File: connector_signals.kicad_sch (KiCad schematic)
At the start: 5 parts, among them J4 Conn_01x05, J5 Conn_01x05, J6 Conn_01x05, J7 Mega Connector/Breakout (if w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, P1 USB_C_Plug_USB2.0

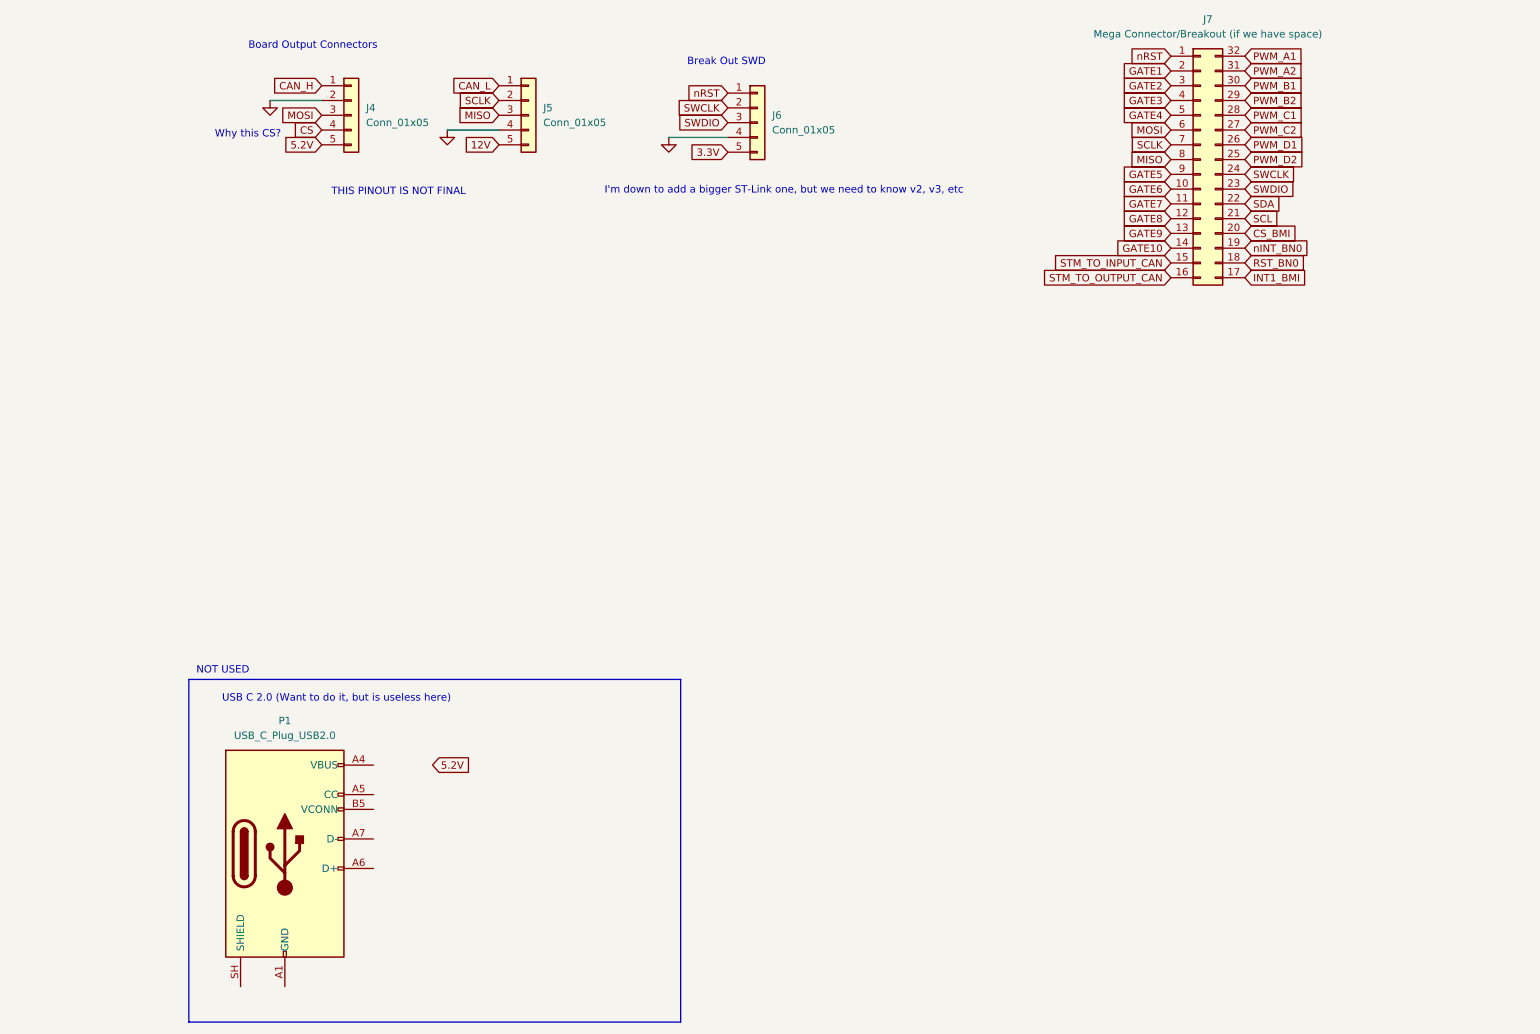
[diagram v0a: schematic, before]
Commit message: Commit for Milwaukee Review
Version 0.2 Completed
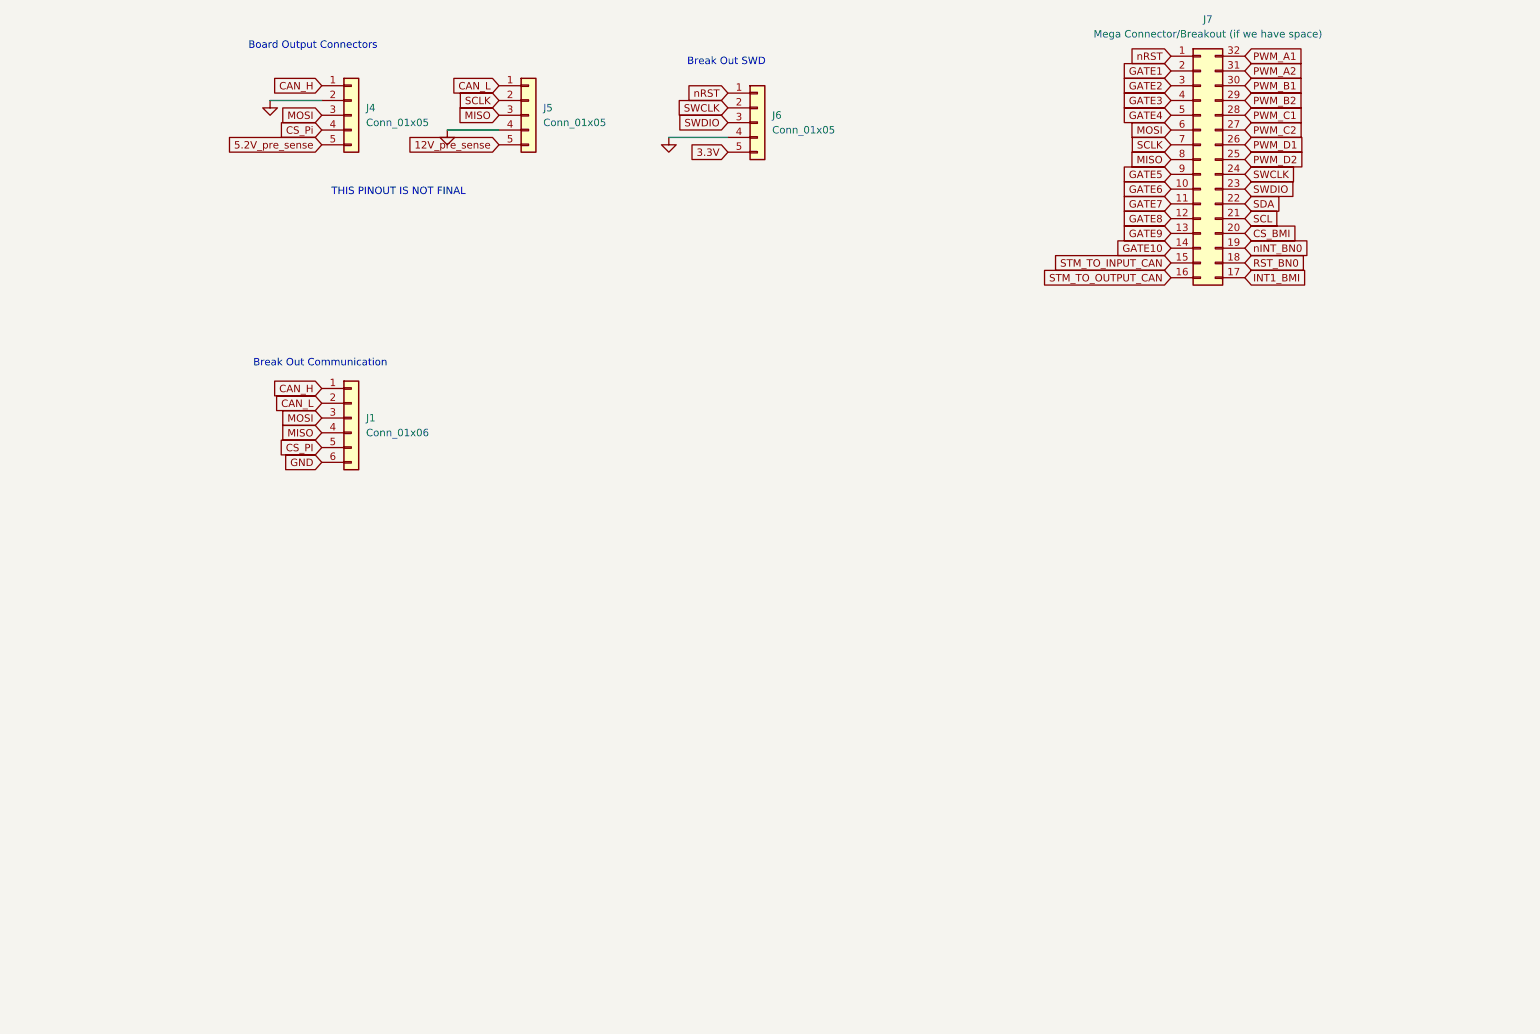
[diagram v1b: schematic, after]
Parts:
- removed P1: USB_C_Plug_USB2.0, symbol Connector:USB_C_Plug_USB2.0
- added J1: Conn_01x06, symbol Connector_Generic:Conn_01x06
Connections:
- net CAN_H: now also J1.1 (Pin_1)
- net CAN_L: now also J1.2 (Pin_2)
- net GND: now also J1.6 (Pin_6)
- net MISO: now also J1.4 (Pin_4)
- net MOSI: now also J1.3 (Pin_3)
- net 12V renamed 12V_pre_sense
- net 5.2V renamed 5.2V_pre_sense
- net CS renamed CS_Pi
- new net CS_PI: J1.5 (Pin_5)
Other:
- note added: "Break Out Communication"
- note removed: "I'm down to add a bigger ST-Link one, but we need to know v2, v3, etc"
- note removed: "NOT USED"
- note removed: "USB C 2.0 (Want to do it, but is useless here)"
- note removed: "Why this CS?"

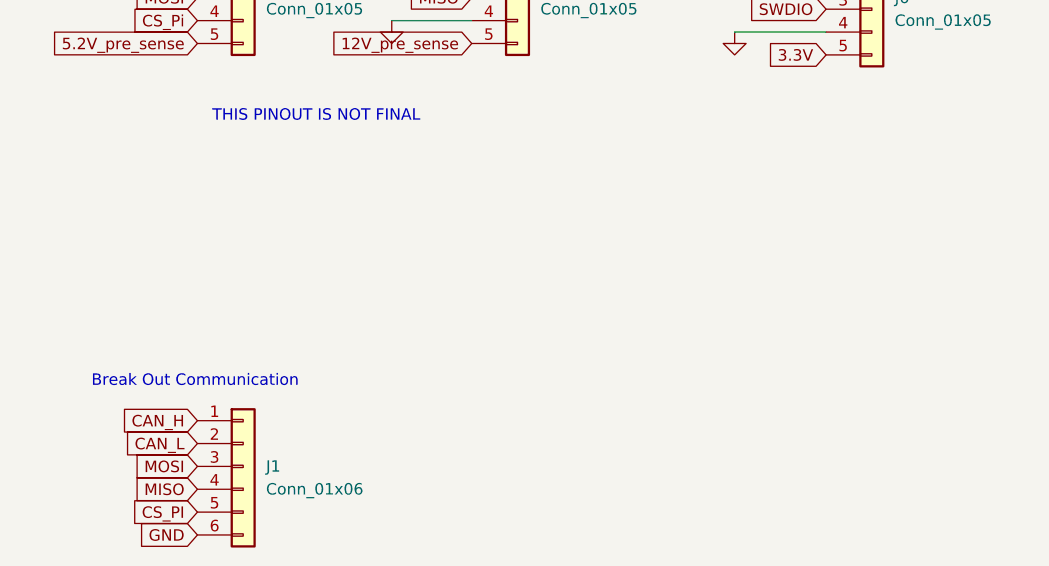
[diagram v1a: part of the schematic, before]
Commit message: Update ig
We messed up
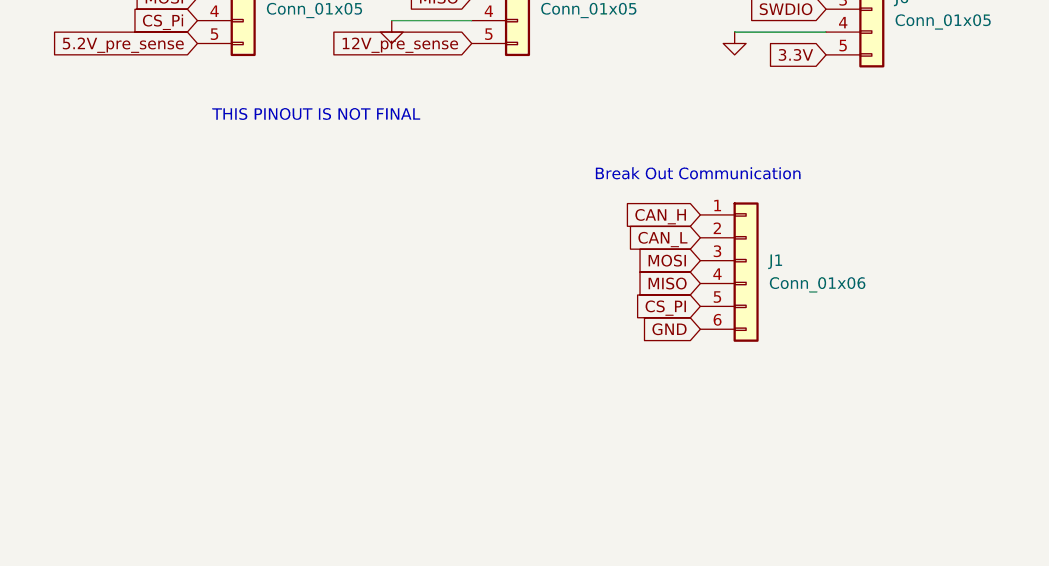
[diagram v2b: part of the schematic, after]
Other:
- moved on the sheet: J1
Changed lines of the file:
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@@
 	(text "Break Out Communication"
 		(exclude_from_sim no)
-		(at 41.656 78.232 0)
+		(at 97.536 55.372 0)
 		(effects
 			(font
@@
 	(global_label "CS_PI"
 		(shape input)
-		(at 41.91 92.71 180)
-		(fields_autoplaced yes)
-		(effects
-			(font
-				(size 1.27 1.27)
-			)
-			(justify right)
-		)
-		(property "Intersheetrefs" "${INTERSHEET_REFS}"
-			(at 33.6029 92.71 0)
+		(at 97.79 69.85 180)
+		(fields_autoplaced yes)
+		(effects
+			(font
+				(size 1.27 1.27)
+			)
+			(justify right)
+		)
+		(property "Intersheetrefs" "${INTERSHEET_REFS}"
+			(at 89.4829 69.85 0)
 			(hide yes)
 			(show_name no)
@@
 	(global_label "GND"
 		(shape input)
-		(at 41.91 95.25 180)
-		(fields_autoplaced yes)
-		(effects
-			(font
-				(size 1.27 1.27)
-			)
-			(justify right)
-		)
-		(property "Intersheetrefs" "${INTERSHEET_REFS}"
-			(at 35.0543 95.25 0)
+		(at 97.79 72.39 180)
+		(fields_autoplaced yes)
+		(effects
+			(font
+				(size 1.27 1.27)
+			)
+			(justify right)
+		)
+		(property "Intersheetrefs" "${INTERSHEET_REFS}"
+			(at 90.9343 72.39 0)
 			(hide yes)
 			(show_name no)
@@
 	(global_label "CAN_L"
 		(shape input)
-		(at 41.91 85.09 180)
-		(fields_autoplaced yes)
-		(effects
-			(font
-				(size 1.27 1.27)
-			)
-			(justify right)
-		)
-		(property "Intersheetrefs" "${INTERSHEET_REFS}"
-			(at 33.24 85.09 0)
+		(at 97.79 62.23 180)
+		(fields_autoplaced yes)
+		(effects
+			(font
+				(size 1.27 1.27)
+			)
+			(justify right)
+		)
+		(property "Intersheetrefs" "${INTERSHEET_REFS}"
+			(at 89.12 62.23 0)
 			(hide yes)
 			(show_name no)
@@
 	(global_label "CAN_H"
 		(shape input)
-		(at 41.91 82.55 180)
-		(fields_autoplaced yes)
-		(effects
-			(font
-				(size 1.27 1.27)
-			)
-			(justify right)
-		)
-		(property "Intersheetrefs" "${INTERSHEET_REFS}"
-			(at 32.9376 82.55 0)
+		(at 97.79 59.69 180)
+		(fields_autoplaced yes)
+		(effects
+			(font
+				(size 1.27 1.27)
+			)
+			(justify right)
+		)
+		(property "Intersheetrefs" "${INTERSHEET_REFS}"
+			(at 88.8176 59.69 0)
 			(hide yes)
 			(show_name no)
@@
 	(global_label "MOSI"
 		(shape input)
-		(at 41.91 87.63 180)
-		(fields_autoplaced yes)
-		(effects
-			(font
-				(size 1.27 1.27)
-			)
-			(justify right)
-		)
-		(property "Intersheetrefs" "${INTERSHEET_REFS}"
-			(at 34.3286 87.63 0)
+		(at 97.79 64.77 180)
+		(fields_autoplaced yes)
+		(effects
+			(font
+				(size 1.27 1.27)
+			)
+			(justify right)
+		)
+		(property "Intersheetrefs" "${INTERSHEET_REFS}"
+			(at 90.2086 64.77 0)
 			(hide yes)
 			(show_name no)
@@
 	(global_label "MISO"
 		(shape input)
-		(at 41.91 90.17 180)
-		(fields_autoplaced yes)
-		(effects
-			(font
-				(size 1.27 1.27)
-			)
-			(justify right)
-		)
-		(property "Intersheetrefs" "${INTERSHEET_REFS}"
-			(at 34.3286 90.17 0)
+		(at 97.79 67.31 180)
+		(fields_autoplaced yes)
+		(effects
+			(font
+				(size 1.27 1.27)
+			)
+			(justify right)
+		)
+		(property "Intersheetrefs" "${INTERSHEET_REFS}"
+			(at 90.2086 67.31 0)
 			(hide yes)
 			(show_name no)
@@
 	(symbol
 		(lib_id "Connector_Generic:Conn_01x06")
-		(at 46.99 87.63 0)
+		(at 102.87 64.77 0)
 		(unit 1)
 		(body_style 1)
@@
 		(fields_autoplaced yes)
 		(property "Reference" "J1"
-			(at 49.53 87.6299 0)
+			(at 105.41 64.7699 0)
 			(show_name no)
 			(do_not_autoplace no)
@@
 		)
 		(property "Value" "Conn_01x06"
-			(at 49.53 90.1699 0)
+			(at 105.41 67.3099 0)
 			(show_name no)
 			(do_not_autoplace no)
@@
 		)
 		(property "Footprint" ""
-			(at 46.99 87.63 0)
+			(at 102.87 64.77 0)
 			(hide yes)
 			(show_name no)
@@
 		)
 		(property "Datasheet" ""
-			(at 46.99 87.63 0)
+			(at 102.87 64.77 0)
 			(hide yes)
 			(show_name no)
@@
 		)
 		(property "Description" "Generic connector, single row, 01x06, script generated (kicad-library-utils/schlib/autogen/connector/)"
-			(at 46.99 87.63 0)
-			(hide yes)
-			(show_name no)
+			(at 102.87 64.77 0)
+			(hide yes)
+			(show_name no)

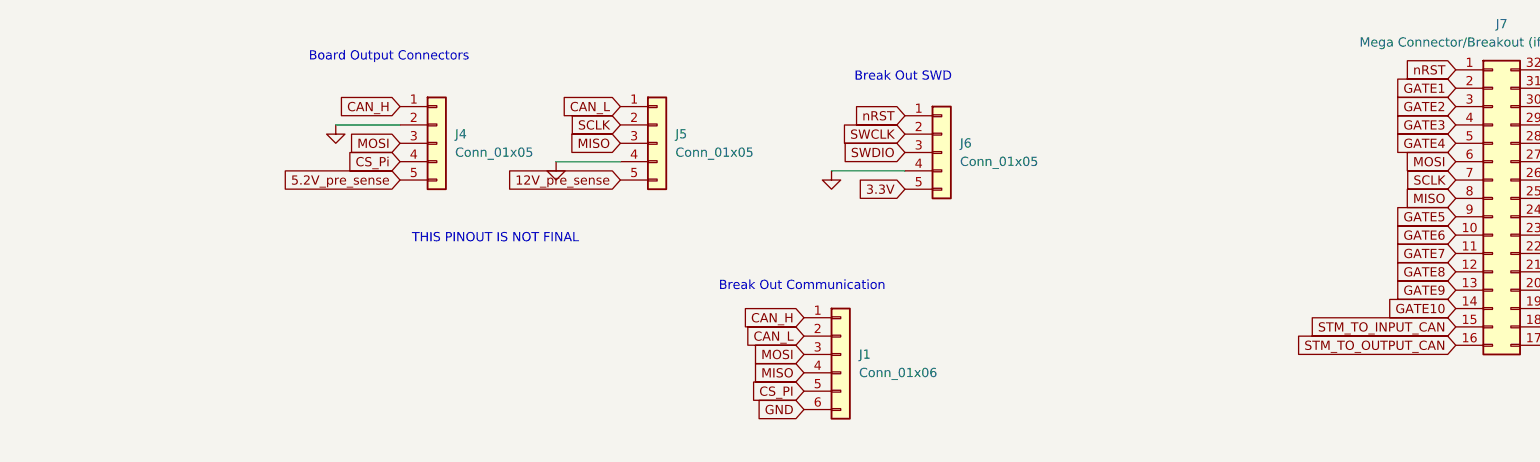
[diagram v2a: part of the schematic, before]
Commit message: 10/14
Fixing my breakout is the only thing... then we can go onto layout
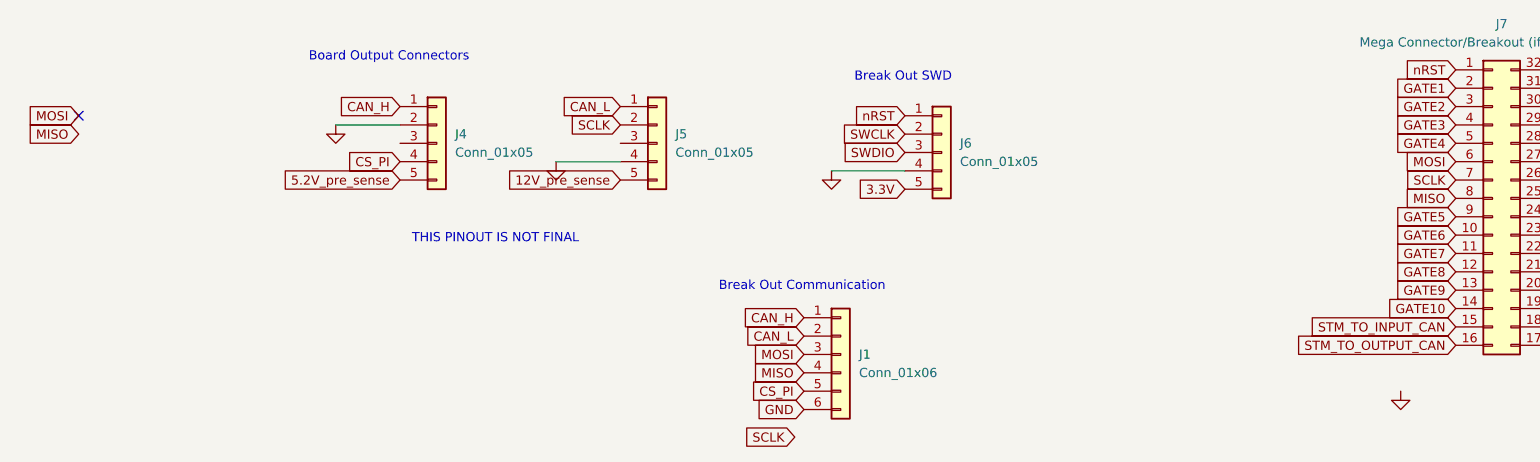
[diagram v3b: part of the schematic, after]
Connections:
- net CS_Pi is gone; now on net CS_PI: J4.4 (Pin_4)
- net MISO: no longer J5.3 (Pin_3)
- net MOSI: no longer J4.3 (Pin_3)
- no-connect marks 0 -> 1
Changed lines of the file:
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@@
 		)
+	)
+	(no_connect
+		(at -2.54 31.75)
 	)
 	(wire
@@
 		)
 	)
+	(global_label "SCLK"
+		(shape input)
+		(at 96.52 76.2 180)
+		(fields_autoplaced yes)
+		(effects
+			(font
+				(size 1.27 1.27)
+			)
+			(justify right)
+		)
+		(property "Intersheetrefs" "${INTERSHEET_REFS}"
+			(at 88.7572 76.2 0)
+			(hide yes)
+			(show_name no)
+			(do_not_autoplace no)
+			(effects
+				(font
+					(size 1.27 1.27)
+				)
+				(justify right)
+			)
+		)
+	)
+	(global_label "MISO"
+		(shape input)
+		(at -2.54 34.29 180)
+		(fields_autoplaced yes)
+		(effects
+			(font
+				(size 1.27 1.27)
+			)
+			(justify right)
+		)
+		(property "Intersheetrefs" "${INTERSHEET_REFS}"
+			(at -10.1214 34.29 0)
+			(hide yes)
+			(show_name no)
+			(do_not_autoplace no)
+			(effects
+				(font
+					(size 1.27 1.27)
+				)
+				(justify right)
+			)
+		)
+	)
 	(global_label "PWM_C2"
 		(shape input)
@@
 		)
 	)
+	(global_label "GATE10"
+		(shape input)
+		(at 187.96 58.42 180)
+		(fields_autoplaced yes)
+		(effects
+			(font
+				(size 1.27 1.27)
+			)
+			(justify right)
+		)
+		(property "Intersheetrefs" "${INTERSHEET_REFS}"
+			(at 178.0806 58.42 0)
+			(hide yes)
+			(show_name no)
+			(do_not_autoplace no)
+			(effects
+				(font
+					(size 1.27 1.27)
+				)
+				(justify right)
+			)
+		)
+	)
 	(global_label "MISO"
 		(shape input)
-		(at 72.39 35.56 180)
-		(fields_autoplaced yes)
-		(effects
-			(font
-				(size 1.27 1.27)
-			)
-			(justify right)
-		)
-		(property "Intersheetrefs" "${INTERSHEET_REFS}"
-			(at 64.8086 35.56 0)
-			(hide yes)
-			(show_name no)
-			(do_not_autoplace no)
-			(effects
-				(font
-					(size 1.27 1.27)
-				)
-				(justify right)
-			)
-		)
-	)
-	(global_label "GATE10"
-		(shape input)
-		(at 187.96 58.42 180)
-		(fields_autoplaced yes)
-		(effects
-			(font
-				(size 1.27 1.27)
-			)
-			(justify right)
-		)
-		(property "Intersheetrefs" "${INTERSHEET_REFS}"
-			(at 178.0806 58.42 0)
-			(hide yes)
-			(show_name no)
-			(do_not_autoplace no)
-			(effects
-				(font
-					(size 1.27 1.27)
-				)
-				(justify right)
-			)
-		)
-	)
-	(global_label "MISO"
-		(shape input)
 		(at 187.96 43.18 180)
 		(fields_autoplaced yes)
@@
 	(global_label "MOSI"
 		(shape input)
-		(at 41.91 35.56 180)
-		(fields_autoplaced yes)
-		(effects
-			(font
-				(size 1.27 1.27)
-			)
-			(justify right)
-		)
-		(property "Intersheetrefs" "${INTERSHEET_REFS}"
-			(at 34.3286 35.56 0)
+		(at -2.54 31.75 180)
+		(fields_autoplaced yes)
+		(effects
+			(font
+				(size 1.27 1.27)
+			)
+			(justify right)
+		)
+		(property "Intersheetrefs" "${INTERSHEET_REFS}"
+			(at -10.1214 31.75 0)
 			(hide yes)
 			(show_name no)
@@
 		)
 	)
-	(global_label "CS_Pi"
+	(global_label "CS_PI"
 		(shape input)
 		(at 41.91 38.1 180)
@@
 					(unit 1)
 				)
+			)
+		)
+	)
+	(symbol
+		(lib_id "power:GND")
+		(at 180.34 69.85 0)
+		(unit 1)
+		(body_style 1)
+		(exclude_from_sim no)
+		(in_bom yes)
+		(on_board yes)
+		(in_pos_files yes)
+		(dnp no)
+		(fields_autoplaced yes)
+		(property "Reference" "#PWR059"
+			(at 180.34 76.2 0)
+			(hide yes)
+			(show_name no)
+			(do_not_autoplace no)
+			(effects
+				(font
+					(size 1.27 1.27)
+				)
+			)
+		)
+		(property "Value" "GND"
+			(at 180.34 74.93 0)
+			(hide yes)
+			(show_name no)
+			(do_not_autoplace no)
+			(effects
+				(font
+					(size 1.27 1.27)
+				)
+			)
+		)
+		(property "Footprint" ""
+			(at 180.34 69.85 0)
+			(hide yes)
+			(show_name no)
+			(do_not_autoplace no)
+			(effects
+				(font
+					(size 1.27 1.27)
+				)
+			)
+		)
+		(property "Datasheet" ""
+			(at 180.34 69.85 0)
+			(hide yes)
+			(show_name no)
+			(do_not_autoplace no)
+			(effects
+				(font
+					(size 1.27 1.27)
+				)
+			)
+		)
+		(property "Description" "Power symbol creates a global label with name \"GND\" , ground"
+			(at 180.34 69.85 0)
+			(hide yes)
+			(show_name no)
+			(do_not_autoplace no)
+			(effects
+				(font
+					(size 1.27 1.27)
+				)
+			)
+		)
+		(pin "1"
+		)
+		(instances
+			(project "X19-Control-Board"
+				(path "/00000000-0000-0000-0000-000060e6118b/5aebb1ae-5eca-4b0a-af28-23512fd077fb"
+					(reference "#PWR059")
+					(unit 1)
+				)
